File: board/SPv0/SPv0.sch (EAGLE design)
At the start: 39 parts, among them IC1 S34ML0XG1, IC2 F55[0/1]X---PT48, IC4 74LS14D, Q1 12MHz

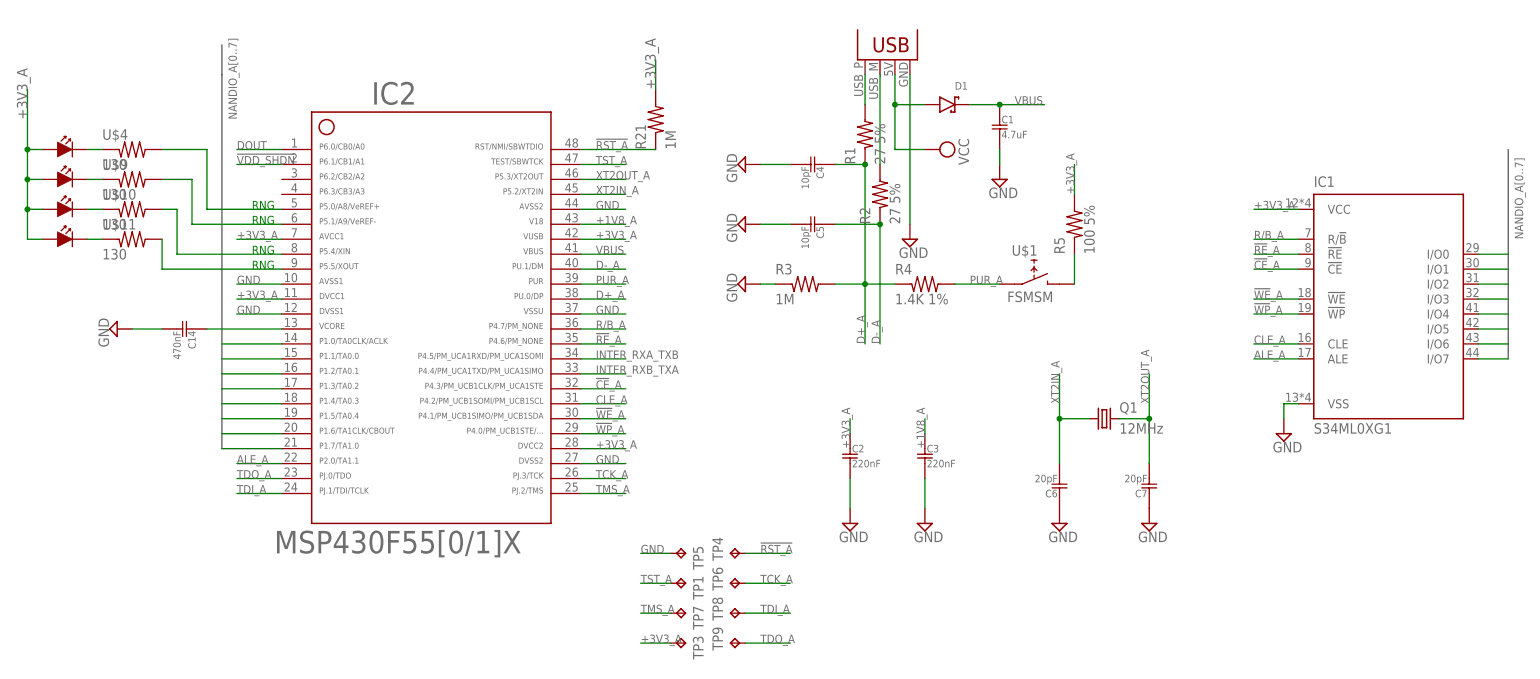
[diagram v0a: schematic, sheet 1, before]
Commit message: halfboard v1 done!
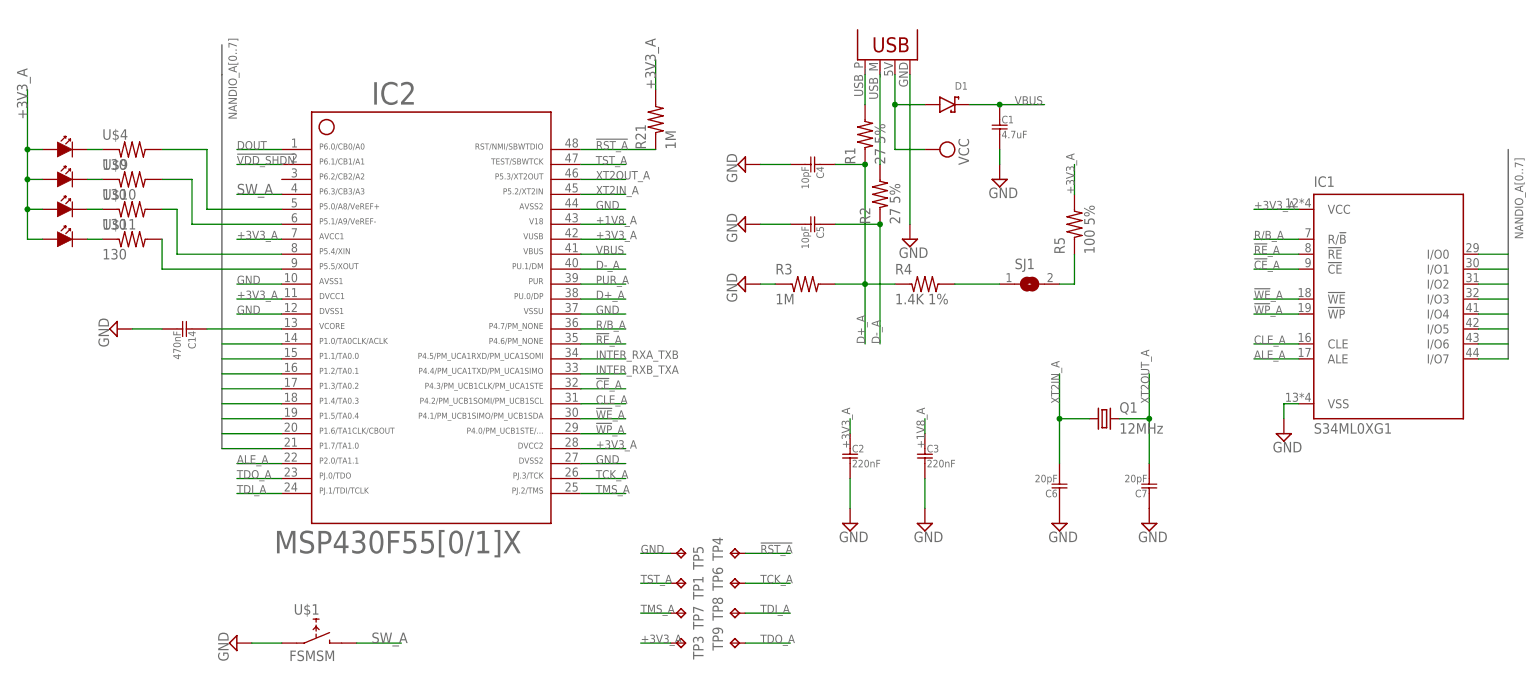
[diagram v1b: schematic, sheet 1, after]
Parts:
- added SJ1: (no value), jumper:SJW
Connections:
- new net N$11: R4.2, SJ1.1
- new net SW_A: IC2.4, U$1.B
- net GND: now also U$1.A1
- net N$4: now also SJ1.2; no longer U$1.B
- net PUR_A: no longer R4.2, U$1.A1
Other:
- note removed: "RNG"
- moved on the sheet: U$1
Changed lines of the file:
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@@
 <part name="R7" library="Passives" deviceset="R" device="0805" value="1.4k"/>
 <part name="SUPPLY13" library="supply2" deviceset="GND" device=""/>
+<part name="SJ1" library="jumper" deviceset="SJ" device="W"/>
+<part name="SUPPLY14" library="supply2" deviceset="GND" device=""/>
 </parts>
 <sheets>
 <sheet>
 <plain>
-<text x="17.78" y="99.06" size="1.4224" layer="91">RNG</text>
-<text x="17.78" y="96.52" size="1.4224" layer="91">RNG</text>
-<text x="17.78" y="106.68" size="1.4224" layer="91">RNG</text>
-<text x="17.78" y="104.14" size="1.4224" layer="91">RNG</text>
 </plain>
 <instances>
@@
 <instance part="R2" gate="G$1" x="124.46" y="109.22" rot="R90"/>
 <instance part="Q1" gate="G$1" x="162.56" y="71.12"/>
-<instance part="U$1" gate="G$1" x="149.86" y="96.52"/>
+<instance part="U$1" gate="G$1" x="27.94" y="35.56"/>
 <instance part="R3" gate="G$1" x="111.76" y="93.98"/>
 <instance part="SUPPLY10" gate="GND" x="101.6" y="93.98" rot="R270"/>
@@
 <instance part="U$11" gate="G$1" x="-2.54" y="101.6"/>
 <instance part="D1" gate="G$1" x="137.16" y="124.46"/>
+<instance part="SJ1" gate="1" x="149.86" y="93.98"/>
+<instance part="SUPPLY14" gate="GND" x="15.24" y="33.02" rot="R270"/>
 </instances>
 <busses>
@@
 <pinref part="C14" gate="G$1" pin="2"/>
 <wire x1="-2.54" y1="86.36" x2="2.54" y2="86.36" width="0.1524" layer="91"/>
+</segment>
+<segment>
+<pinref part="SUPPLY14" gate="GND" pin="GND"/>
+<pinref part="U$1" gate="G$1" pin="A1"/>
+<wire x1="17.78" y1="33.02" x2="22.86" y2="33.02" width="0.1524" layer="91"/>
 </segment>
 </net>
@@
 <label x="76.2" y="93.98" size="1.4224" layer="95"/>
 </segment>
-<segment>
-<pinref part="R4" gate="G$1" pin="2"/>
-<pinref part="U$1" gate="G$1" pin="A1"/>
-<wire x1="137.16" y1="93.98" x2="144.78" y2="93.98" width="0.1524" layer="91"/>
-<label x="139.7" y="93.98" size="1.4224" layer="95"/>
-</segment>
-</net>
-<net name="N$4" class="0">
-<segment>
-<pinref part="U$1" gate="G$1" pin="B"/>
-<pinref part="R5" gate="G$1" pin="1"/>
-<wire x1="157.48" y1="93.98" x2="157.48" y2="99.06" width="0.1524" layer="91"/>
-</segment>
 </net>
 <net name="TDO_A" class="0">
@@
 </segment>
 </net>
+<net name="N$4" class="0">
+<segment>
+<pinref part="R5" gate="G$1" pin="1"/>
+<wire x1="157.48" y1="99.06" x2="157.48" y2="93.98" width="0.1524" layer="91"/>
+<pinref part="SJ1" gate="1" pin="2"/>
+<wire x1="157.48" y1="93.98" x2="154.94" y2="93.98" width="0.1524" layer="91"/>
+</segment>
+</net>
+<net name="N$11" class="0">
+<segment>
+<pinref part="SJ1" gate="1" pin="1"/>
+<pinref part="R4" gate="G$1" pin="2"/>
+<wire x1="144.78" y1="93.98" x2="137.16" y2="93.98" width="0.1524" layer="91"/>
+</segment>
+</net>
+<net name="SW_A" class="0">
+<segment>
+<pinref part="U$1" gate="G$1" pin="B"/>
+<wire x1="35.56" y1="33.02" x2="43.18" y2="33.02" width="0.1524" layer="91"/>
+<label x="38.1" y="33.02" size="1.778" layer="95"/>
+</segment>
+<segment>
+<pinref part="IC2" gate="G$1" pin="4"/>
+<wire x1="22.86" y1="109.22" x2="15.24" y2="109.22" width="0.1524" layer="91"/>
+<label x="15.24" y="109.22" size="1.778" layer="95"/>
+</segment>
+</net>
